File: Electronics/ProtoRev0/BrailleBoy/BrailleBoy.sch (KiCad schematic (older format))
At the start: 33 parts, among them SW1 B0, SW2 B1, SW3 B2, SW4 B3, SW5 RESET, U1 MCP23S17, U2 SPH0645-BRK-ADAFRUIT, U3 ESP32-WROOM

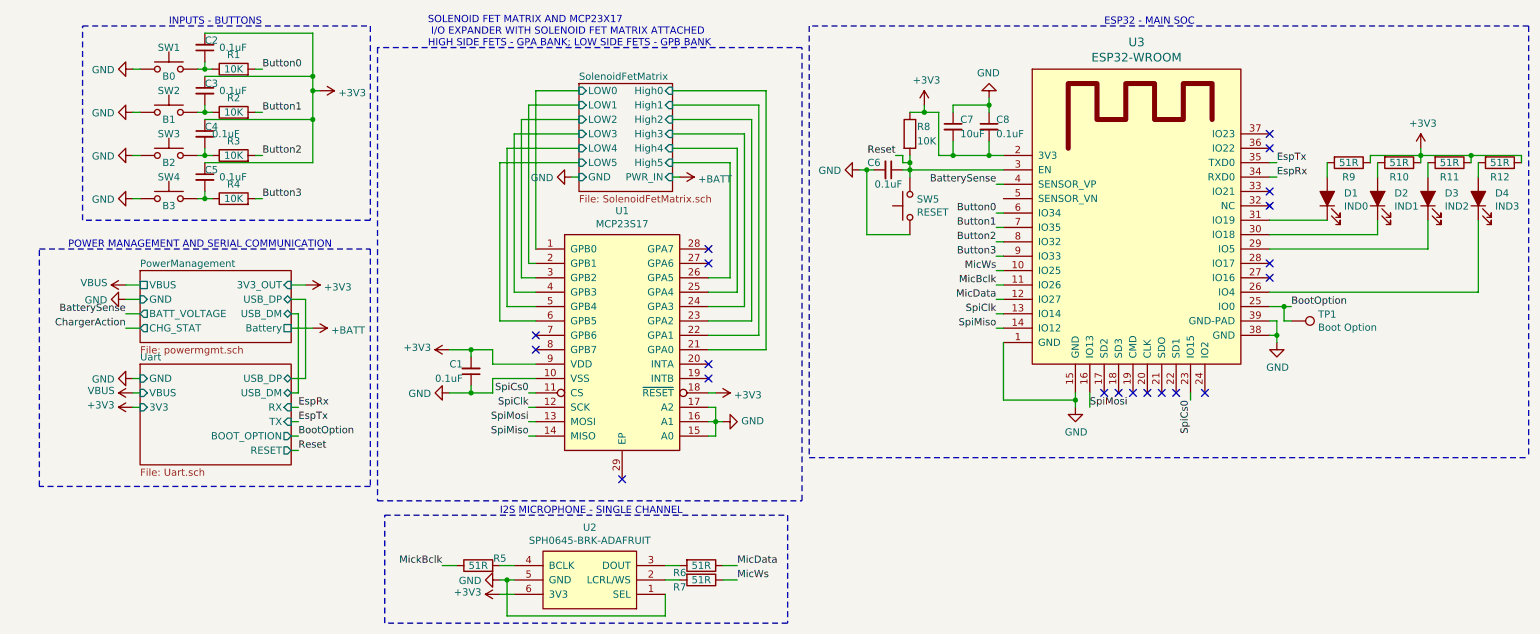
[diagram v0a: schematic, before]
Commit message: Made the schematic sheets a bit prettier
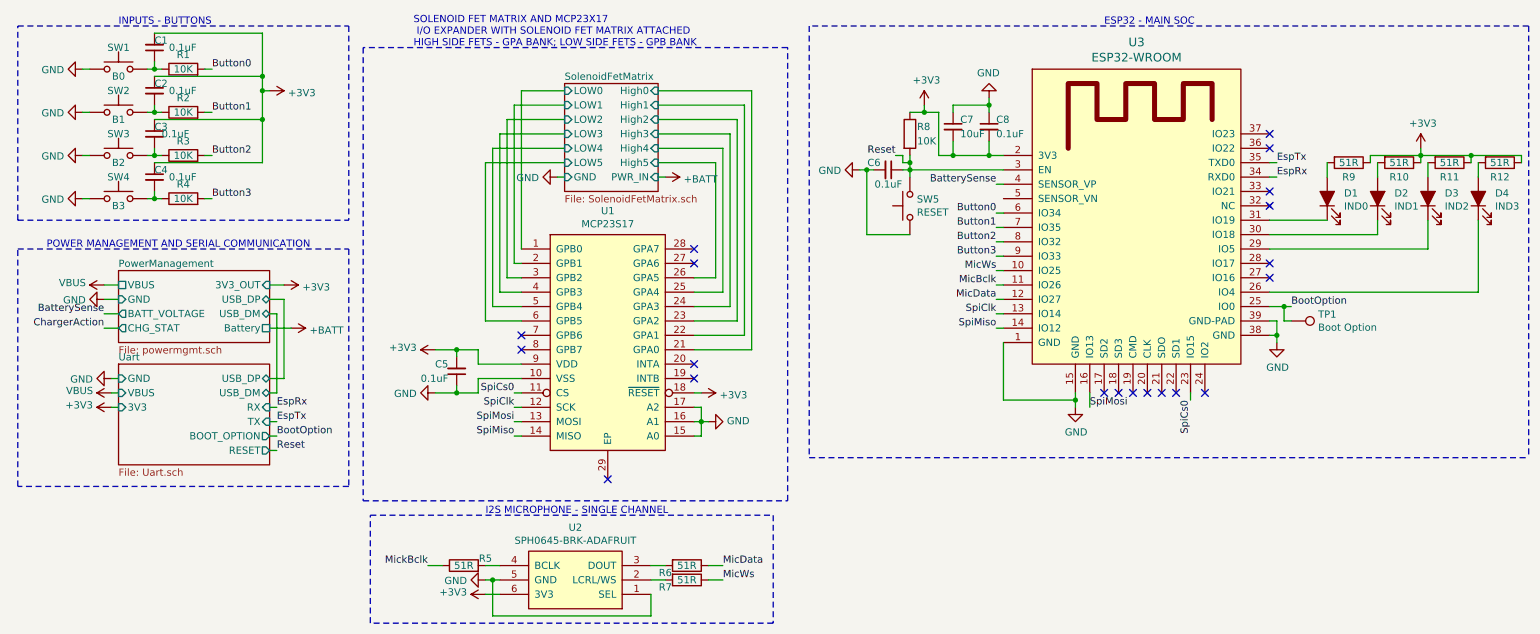
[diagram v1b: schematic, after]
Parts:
- renumbered C2 to C1, C3 to C2, C4 to C3, C5 to C4, C1 to C5
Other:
- moved on the sheet: C1, C2, C3, C4, C5, R1, R2, R3, R4, R5, R6, R7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
